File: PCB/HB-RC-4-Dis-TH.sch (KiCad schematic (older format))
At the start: 59 parts, among them J3 eInk, J5 Power, J6 Batt, Q1 IRLML6346TRBPF, SW1 T1, SW2 T2, SW3 T3, SW4 T4, SW5 Config, U1 ATmega1284P-AU, U2 CC1101, U3 MCP1703T-3302E/CB, U4 MCP73831T-2ACI/OT, U5 PC357

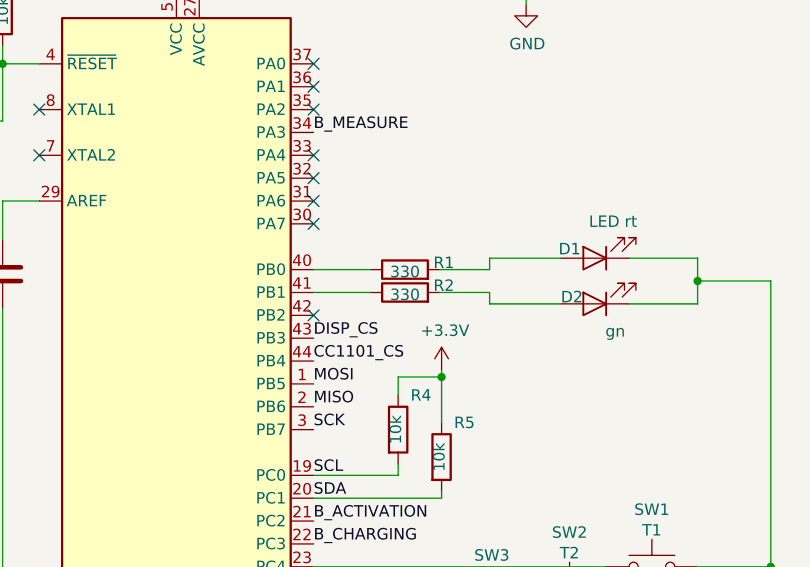
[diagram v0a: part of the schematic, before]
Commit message: update pcb
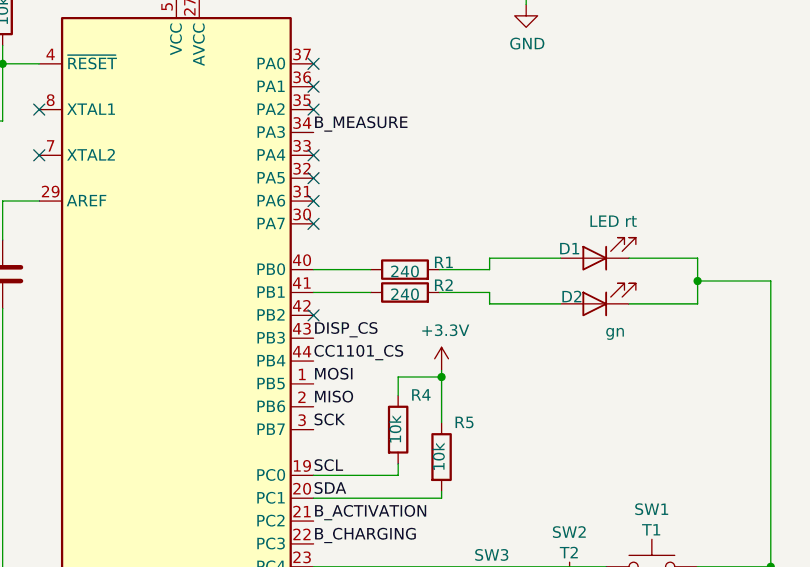
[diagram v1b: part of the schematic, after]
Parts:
- R1, R2: value 330 -> 240
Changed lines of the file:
@@
 P 8850 2750
 F 0 "R1" V 8880 2580 50  0000 C CNN
-F 1 "330" V 8840 2750 50  0000 C CNN
+F 1 "240" V 8840 2750 50  0000 C CNN
 F 2 "Resistor_SMD:R_0805_2012Metric_Pad1.15x1.40mm_HandSolder" V 8780 2750 50  0001 C CNN
 F 3 "~" H 8850 2750 50  0001 C CNN
@@
 P 8850 2850
 F 0 "R2" V 8880 2680 50  0000 C CNN
-F 1 "330" V 8840 2850 50  0000 C CNN
+F 1 "240" V 8840 2850 50  0000 C CNN
 F 2 "Resistor_SMD:R_0805_2012Metric_Pad1.15x1.40mm_HandSolder" V 8780 2850 50  0001 C CNN
 F 3 "~" H 8850 2850 50  0001 C CNN
